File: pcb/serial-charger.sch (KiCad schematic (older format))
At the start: 5 parts, among them P102 CONN_01X02, P103 CONN_01X04

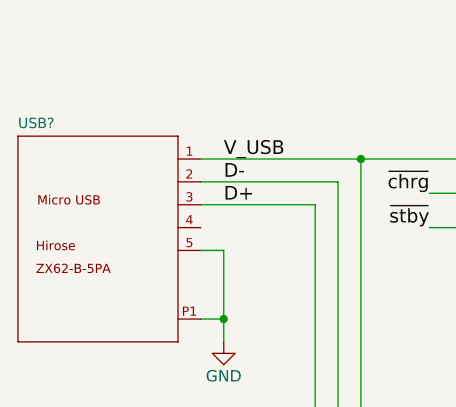
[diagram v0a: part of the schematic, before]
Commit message: layout mostly done
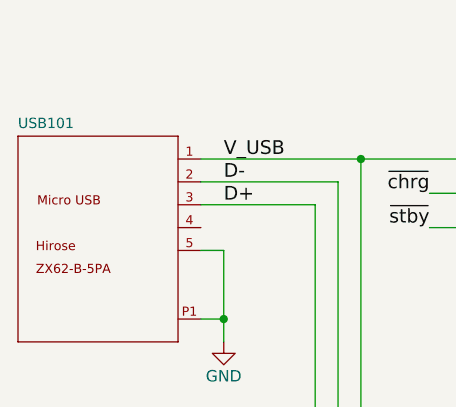
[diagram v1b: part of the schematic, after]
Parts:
- gave numbers to parts that had none: 1
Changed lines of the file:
@@
 $EndDescr
 $Comp
-L GND #PWR01
+L GND #PWR101
 U 1 1 55AEBF75
 P 2300 3500
-F 0 "#PWR01" H 2300 3250 50  0001 C CNN
+F 0 "#PWR101" H 2300 3250 50  0001 C CNN
 F 1 "GND" H 2300 3350 50  0000 C CNN
 F 2 "" H 2300 3500 60  0000 C CNN
@@
 	2200 2800 2800 2800
 $Comp
-L GND #PWR02
+L GND #PWR102
 U 1 1 57F8F41D
 P 5200 3300
-F 0 "#PWR02" H 5200 3050 50  0001 C CNN
+F 0 "#PWR102" H 5200 3050 50  0001 C CNN
 F 1 "GND" H 5200 3150 50  0000 C CNN
 F 2 "" H 5200 3300 60  0000 C CNN
@@
 $EndSheet
 $Comp
-L GND #PWR03
+L GND #PWR104
 U 1 1 58B9EA67
 P 7900 5500
-F 0 "#PWR03" H 7900 5250 50  0001 C CNN
+F 0 "#PWR104" H 7900 5250 50  0001 C CNN
 F 1 "GND" H 7900 5350 50  0000 C CNN
 F 2 "" H 7900 5500 50  0000 C CNN
@@
 	5850 4950 5850 4550
 $Comp
-L GND #PWR04
+L GND #PWR103
 U 1 1 58BACB26
 P 5950 4700
-F 0 "#PWR04" H 5950 4450 50  0001 C CNN
+F 0 "#PWR103" H 5950 4450 50  0001 C CNN
 F 1 "GND" H 5950 4550 50  0000 C CNN
 F 2 "" H 5950 4700 50  0000 C CNN
@@
 	6800 2950 6700 2950
 $Comp
-L MICRO-USB-SMD_ZX62-B-5PA_ USB?
+L MICRO-USB-SMD_ZX62-B-5PA_ USB101
 U 1 1 5A559483
 P 1800 3100
-F 0 "USB?" H 1400 3630 45  0000 L BNN
+F 0 "USB101" H 1400 3630 45  0000 L BNN
 F 1 "MICRO-USB-SMD_ZX62-B-5PA_" H 1800 3100 45  0001 L BNN
 F 2 "SeeedOPL-Connector-2016:MICRO-USB5+4P-SMD-0.65-B" H 1800 3100 60  0001 C CNN
